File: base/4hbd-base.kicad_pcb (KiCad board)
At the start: 2 copper layers, 223 parts, among them J1 Spring_Terminal_Connector_01x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, J10 Spring_Terminal_Connector_01x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, J11 Spring_Terminal_Connector_01x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, J12 Spring_Terminal_Connector_01x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, J13 Screw_Terminal_01x02, J14 Conn_02x25_Odd_Even, J15 Conn_02x25_Odd_Even, J2 Spring_Terminal_Connector_01x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, J3 Spring_Terminal_Connector_01x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, J4 Spring_Terminal_Connector_01x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, J5 Spring_Terminal_Connector_01x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, J6 Spring_Terminal_Connector_01x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, J7 Screw_Terminal_01x03, J8 Spring_Terminal_Connector_01x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, J9 Spring_Terminal_Connector_01x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, Q1 irf540n, Q10 2N7002, Q11 2N7002, Q12 IRLML2060TRPBF, Q2 irf540n, Q3 irf540n, Q4 irf540n, Q5 irf540n, Q6 irf540n, Q7 irf540n, Q8 irf540n, Q9 2N7002, U1 SI8640, U10 ADS7886, U11 MOCD217M, U12 MOCD217M, U13 MOCD217M, U14 AMS1117-5.0, U15 AMS1117-5.0, U16 LM2596S-ADJ, U17 AM26LV32, U18 LM2596S-ADJ, U19 AMS1117-5.0, U2 SI8640, U20 SN65HVD230, U21 MAX485CSA, U3 IR2181, U4 IR2181, U5 IR2181, U6 IR2181, U7 ACS712xLCTR-30A, U8 ACS712xLCTR-30A, U9 ADS7886

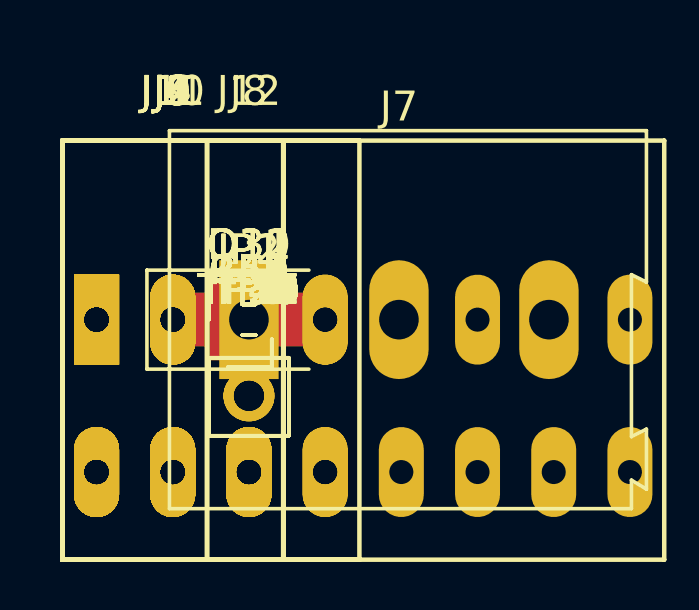
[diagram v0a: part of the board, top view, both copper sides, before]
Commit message: assign footprints
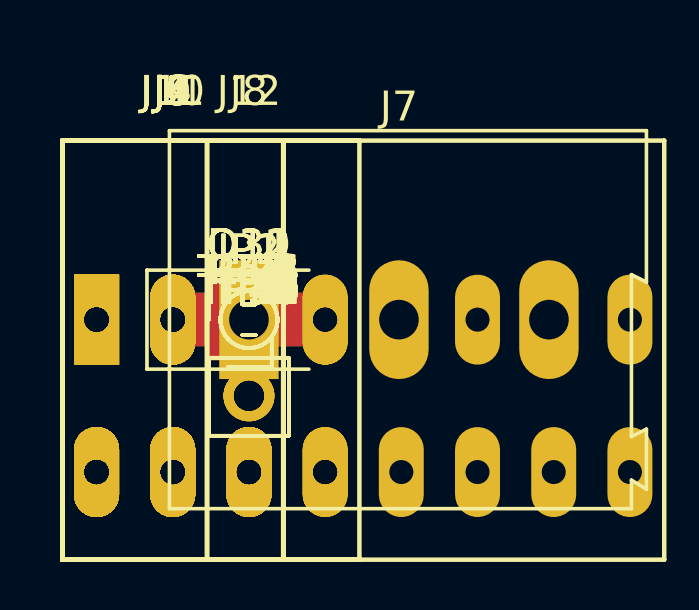
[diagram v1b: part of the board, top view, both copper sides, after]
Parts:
- added TP21: SPI0_sck, TestPoint:TestPoint_Pad_D1.5mm, F.Cu at (0.00, 0.00)
- added TP22: SPI0_cs, TestPoint:TestPoint_Pad_D1.5mm, F.Cu at (0.00, 0.00)
- added TP23: SPI0_miso, TestPoint:TestPoint_Pad_D1.5mm, F.Cu at (0.00, 0.00)
- added TP24: SPI1_sck, TestPoint:TestPoint_Pad_D1.5mm, F.Cu at (0.00, 0.00)
- added TP25: SPI1_cs, TestPoint:TestPoint_Pad_D1.5mm, F.Cu at (0.00, 0.00)
- added TP26: SPI1_miso, TestPoint:TestPoint_Pad_D1.5mm, F.Cu at (0.00, 0.00)
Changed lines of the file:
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@@
 (kicad_pcb (version 4) (host pcbnew 4.0.2+dfsg1-stable)
   (general
-    (links 497)
-    (no_connects 278)
+    (links 503)
+    (no_connects 284)
     (area 0 0 0 0)
     (thickness 1.6)
@@
     (tracks 0)
     (zones 0)
-    (modules 223)
+    (modules 229)
     (nets 193)
   )
@@
     (attr virtual)
     (fp_text reference TP34 (at 0 -1) (layer F.SilkS)
-      (effects (font (size 1 1)))
+      (effects (font (size 1 1) (thickness 0.15)))
     )
     (fp_text value +6.8Vd (at 0 1) (layer F.Fab)
-      (effects (font (size 1 1)))
+      (effects (font (size 1 1) (thickness 0.15)))
     )
     (fp_text user %R (at 0 -1) (layer F.Fab)
-      (effects (font (size 1 1)))
+      (effects (font (size 1 1) (thickness 0.15)))
     )
     (fp_circle (center 0 0) (end 1 0) (layer F.CrtYd) (width 0))
@@
     (attr virtual)
     (fp_text reference TP38 (at 0 -1) (layer F.SilkS)
-      (effects (font (size 1 1)))
+      (effects (font (size 1 1) (thickness 0.15)))
     )
     (fp_text value CAN_Tx (at 0 1) (layer F.Fab)
-      (effects (font (size 1 1)))
+      (effects (font (size 1 1) (thickness 0.15)))
     )
     (fp_text user %R (at 0 -1) (layer F.Fab)
-      (effects (font (size 1 1)))
+      (effects (font (size 1 1) (thickness 0.15)))
     )
     (fp_circle (center 0 0) (end 1 0) (layer F.CrtYd) (width 0))
@@
     (attr virtual)
     (fp_text reference TP39 (at 0 -1) (layer F.SilkS)
-      (effects (font (size 1 1)))
+      (effects (font (size 1 1) (thickness 0.15)))
     )
     (fp_text value CAN_Rx (at 0 1) (layer F.Fab)
-      (effects (font (size 1 1)))
+      (effects (font (size 1 1) (thickness 0.15)))
     )
     (fp_text user %R (at 0 -1) (layer F.Fab)
-      (effects (font (size 1 1)))
+      (effects (font (size 1 1) (thickness 0.15)))
     )
     (fp_circle (center 0 0) (end 1 0) (layer F.CrtYd) (width 0))
@@
     (attr virtual)
     (fp_text reference TP40 (at 0 -1) (layer F.SilkS)
-      (effects (font (size 1 1)))
+      (effects (font (size 1 1) (thickness 0.15)))
     )
     (fp_text value 485_Tx (at 0 1) (layer F.Fab)
-      (effects (font (size 1 1)))
+      (effects (font (size 1 1) (thickness 0.15)))
     )
     (fp_text user %R (at 0 -1) (layer F.Fab)
-      (effects (font (size 1 1)))
+      (effects (font (size 1 1) (thickness 0.15)))
     )
     (fp_circle (center 0 0) (end 1 0) (layer F.CrtYd) (width 0))
@@
     (attr virtual)
     (fp_text reference TP41 (at 0 -1) (layer F.SilkS)
-      (effects (font (size 1 1)))
+      (effects (font (size 1 1) (thickness 0.15)))
     )
     (fp_text value 485_Rx (at 0 1) (layer F.Fab)
-      (effects (font (size 1 1)))
+      (effects (font (size 1 1) (thickness 0.15)))
     )
     (fp_text user %R (at 0 -1) (layer F.Fab)
-      (effects (font (size 1 1)))
+      (effects (font (size 1 1) (thickness 0.15)))
     )
     (fp_circle (center 0 0) (end 1 0) (layer F.CrtYd) (width 0))
@@
     (attr virtual)
     (fp_text reference TP42 (at 0 -1) (layer F.SilkS)
-      (effects (font (size 1 1)))
+      (effects (font (size 1 1) (thickness 0.15)))
     )
     (fp_text value 485_TxEn (at 0 1) (layer F.Fab)
-      (effects (font (size 1 1)))
+      (effects (font (size 1 1) (thickness 0.15)))
     )
     (fp_text user %R (at 0 -1) (layer F.Fab)
-      (effects (font (size 1 1)))
+      (effects (font (size 1 1) (thickness 0.15)))
     )
     (fp_circle (center 0 0) (end 1 0) (layer F.CrtYd) (width 0))
@@
       (net 125 /CAN/RS485/RS485_TXEN))
   )
+  (module TestPoint:TestPoint_Pad_D1.5mm (layer F.Cu)
+    (at 0 0)
+    (descr "SMD pad as test Point, diameter 1.5mm")
+    (tags "test point SMD pad")
+    (attr virtual)
+    (fp_text reference TP21 (at 0 -1.648) (layer F.SilkS)
+      (effects (font (size 1 1) (thickness 0.15)))
+    )
+    (fp_text value SPI0_sck (at 0 1.75) (layer F.Fab)
+      (effects (font (size 1 1) (thickness 0.15)))
+    )
+    (fp_text user %R (at 0 -1.65) (layer F.Fab)
+      (effects (font (size 1 1) (thickness 0.15)))
+    )
+    (fp_circle (center 0 0) (end 1.25 0) (layer F.CrtYd) (width 0.05))
+    (fp_circle (center 0 0) (end 0 0.95) (layer F.SilkS) (width 0.12))
+    (pad 1 smd circle (at 0 0) (size 1.5 1.5) (layers F.Cu F.Mask)
+      (net 72 "/MCU/FPGA connection/SPI0_SCK"))
+  )
+  (module TestPoint:TestPoint_Pad_D1.5mm (layer F.Cu)
+    (at 0 0)
+    (descr "SMD pad as test Point, diameter 1.5mm")
+    (tags "test point SMD pad")
+    (attr virtual)
+    (fp_text reference TP22 (at 0 -1.648) (layer F.SilkS)
+      (effects (font (size 1 1) (thickness 0.15)))
+    )
+    (fp_text value SPI0_cs (at 0 1.75) (layer F.Fab)
+      (effects (font (size 1 1) (thickness 0.15)))
+    )
+    (fp_text user %R (at 0 -1.65) (layer F.Fab)
+      (effects (font (size 1 1) (thickness 0.15)))
+    )
+    (fp_circle (center 0 0) (end 1.25 0) (layer F.CrtYd) (width 0.05))
+    (fp_circle (center 0 0) (end 0 0.95) (layer F.SilkS) (width 0.12))
+    (pad 1 smd circle (at 0 0) (size 1.5 1.5) (layers F.Cu F.Mask)
+      (net 71 "/MCU/FPGA connection/SPI0_CSn"))
+  )
+  (module TestPoint:TestPoint_Pad_D1.5mm (layer F.Cu)
+    (at 0 0)
+    (descr "SMD pad as test Point, diameter 1.5mm")
+    (tags "test point SMD pad")
+    (attr virtual)
+    (fp_text reference TP23 (at 0 -1.648) (layer F.SilkS)
+      (effects (font (size 1 1) (thickness 0.15)))
+    )
+    (fp_text value SPI0_miso (at 0 1.75) (layer F.Fab)
+      (effects (font (size 1 1) (thickness 0.15)))
+    )
+    (fp_text user %R (at 0 -1.65) (layer F.Fab)
+      (effects (font (size 1 1) (thickness 0.15)))
+    )
+    (fp_circle (center 0 0) (end 1.25 0) (layer F.CrtYd) (width 0.05))
+    (fp_circle (center 0 0) (end 0 0.95) (layer F.SilkS) (width 0.12))
+    (pad 1 smd circle (at 0 0) (size 1.5 1.5) (layers F.Cu F.Mask)
+      (net 73 "/MCU/FPGA connection/SPI0_MISO"))
+  )
+  (module TestPoint:TestPoint_Pad_D1.5mm (layer F.Cu)
+    (at 0 0)
+    (descr "SMD pad as test Point, diameter 1.5mm")
+    (tags "test point SMD pad")
+    (attr virtual)
+    (fp_text reference TP24 (at 0 -1.648) (layer F.SilkS)
+      (effects (font (size 1 1) (thickness 0.15)))
+    )
+    (fp_text value SPI1_sck (at 0 1.75) (layer F.Fab)
+      (effects (font (size 1 1) (thickness 0.15)))
+    )
+    (fp_text user %R (at 0 -1.65) (layer F.Fab)
+      (effects (font (size 1 1) (thickness 0.15)))
+    )
+    (fp_circle (center 0 0) (end 1.25 0) (layer F.CrtYd) (width 0.05))
+    (fp_circle (center 0 0) (end 0 0.95) (layer F.SilkS) (width 0.12))
+    (pad 1 smd circle (at 0 0) (size 1.5 1.5) (layers F.Cu F.Mask)
+      (net 90 "/MCU/FPGA connection/SPI1_SCK"))
+  )
+  (module TestPoint:TestPoint_Pad_D1.5mm (layer F.Cu)
+    (at 0 0)
+    (descr "SMD pad as test Point, diameter 1.5mm")
+    (tags "test point SMD pad")
+    (attr virtual)
+    (fp_text reference TP25 (at 0 -1.648) (layer F.SilkS)
+      (effects (font (size 1 1) (thickness 0.15)))
+    )
+    (fp_text value SPI1_cs (at 0 1.75) (layer F.Fab)
+      (effects (font (size 1 1) (thickness 0.15)))
+    )
+    (fp_text user %R (at 0 -1.65) (layer F.Fab)
+      (effects (font (size 1 1) (thickness 0.15)))
+    )
+    (fp_circle (center 0 0) (end 1.25 0) (layer F.CrtYd) (width 0.05))
+    (fp_circle (center 0 0) (end 0 0.95) (layer F.SilkS) (width 0.12))
+    (pad 1 smd circle (at 0 0) (size 1.5 1.5) (layers F.Cu F.Mask)
+      (net 89 "/MCU/FPGA connection/SPI1_CSn"))
+  )
+  (module TestPoint:TestPoint_Pad_D1.5mm (layer F.Cu)
+    (at 0 0)
+    (descr "SMD pad as test Point, diameter 1.5mm")
+    (tags "test point SMD pad")
+    (attr virtual)
+    (fp_text reference TP26 (at 0 -1.648) (layer F.SilkS)
+      (effects (font (size 1 1) (thickness 0.15)))
+    )
+    (fp_text value SPI1_miso (at 0 1.75) (layer F.Fab)
+      (effects (font (size 1 1) (thickness 0.15)))
+    )
+    (fp_text user %R (at 0 -1.65) (layer F.Fab)
+      (effects (font (size 1 1) (thickness 0.15)))
+    )
+    (fp_circle (center 0 0) (end 1.25 0) (layer F.CrtYd) (width 0.05))
+    (fp_circle (center 0 0) (end 0 0.95) (layer F.SilkS) (width 0.12))
+    (pad 1 smd circle (at 0 0) (size 1.5 1.5) (layers F.Cu F.Mask)
+      (net 91 "/MCU/FPGA connection/SPI1_MISO"))
+  )
 )
